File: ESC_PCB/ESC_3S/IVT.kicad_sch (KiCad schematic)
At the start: 45 parts, among them Q1 CSD18532Q5BT, Q2 CSD18532Q5BT, Q3 CSD18532Q5BT, Q4 CSD18532Q5BT, Q5 CSD18532Q5BT, Q6 CSD18532Q5BT, U4 FD6288Q

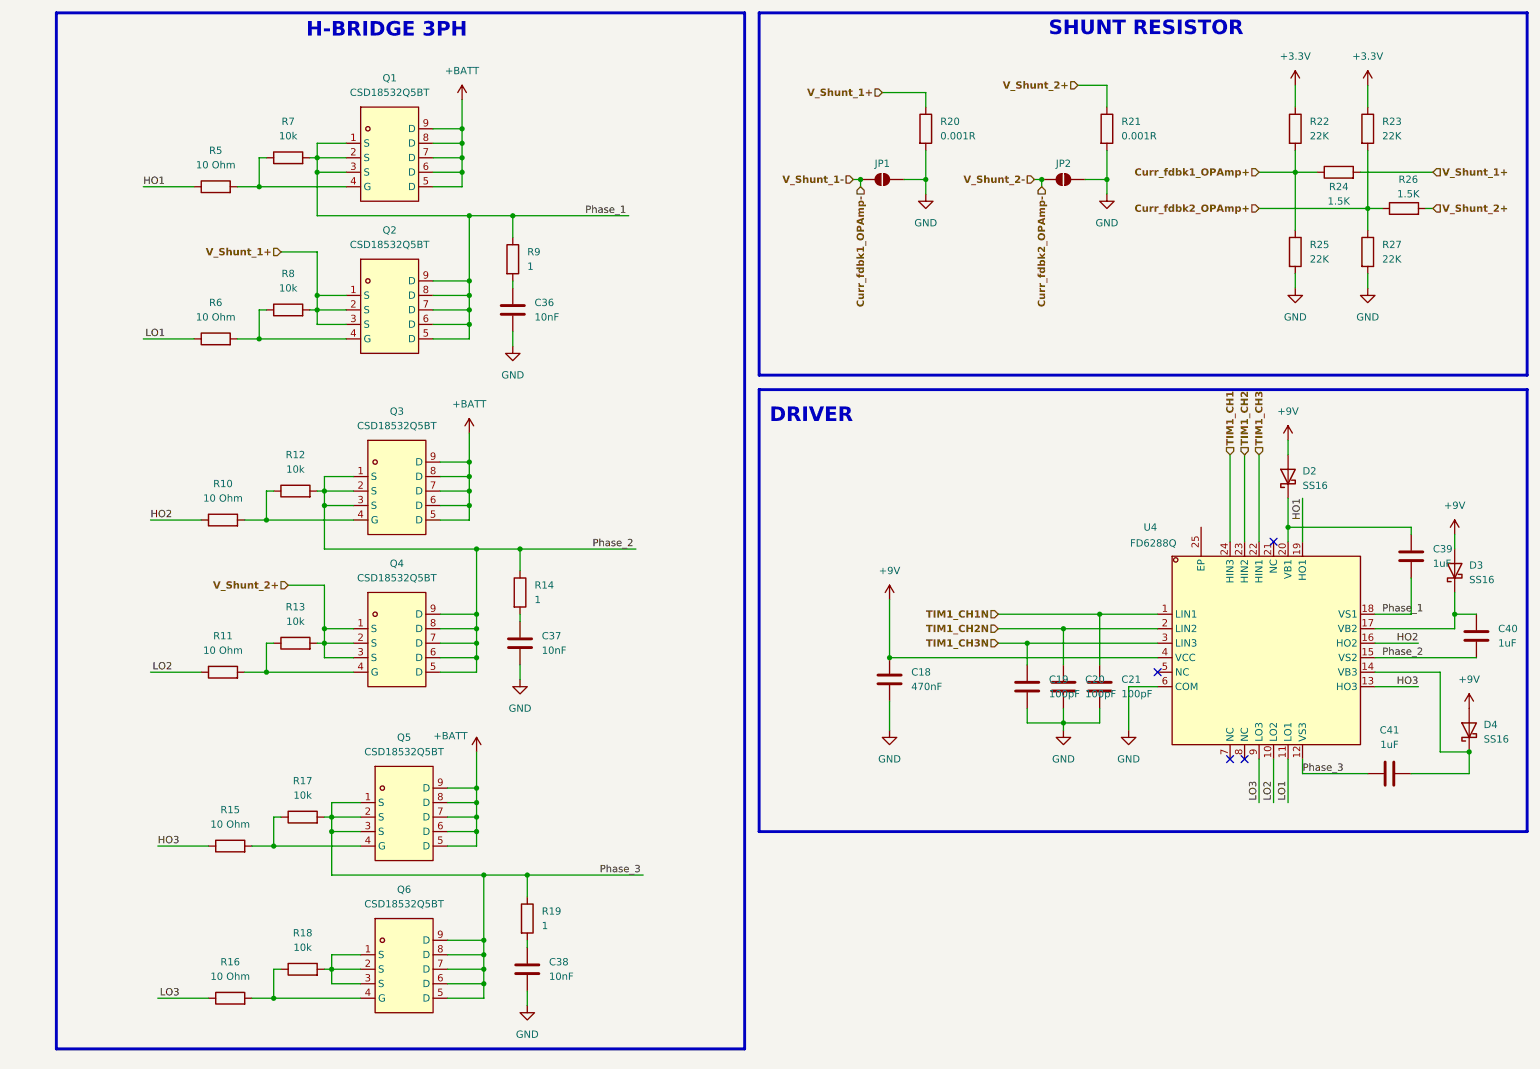
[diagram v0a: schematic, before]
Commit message: add .ioc and temperature done sch
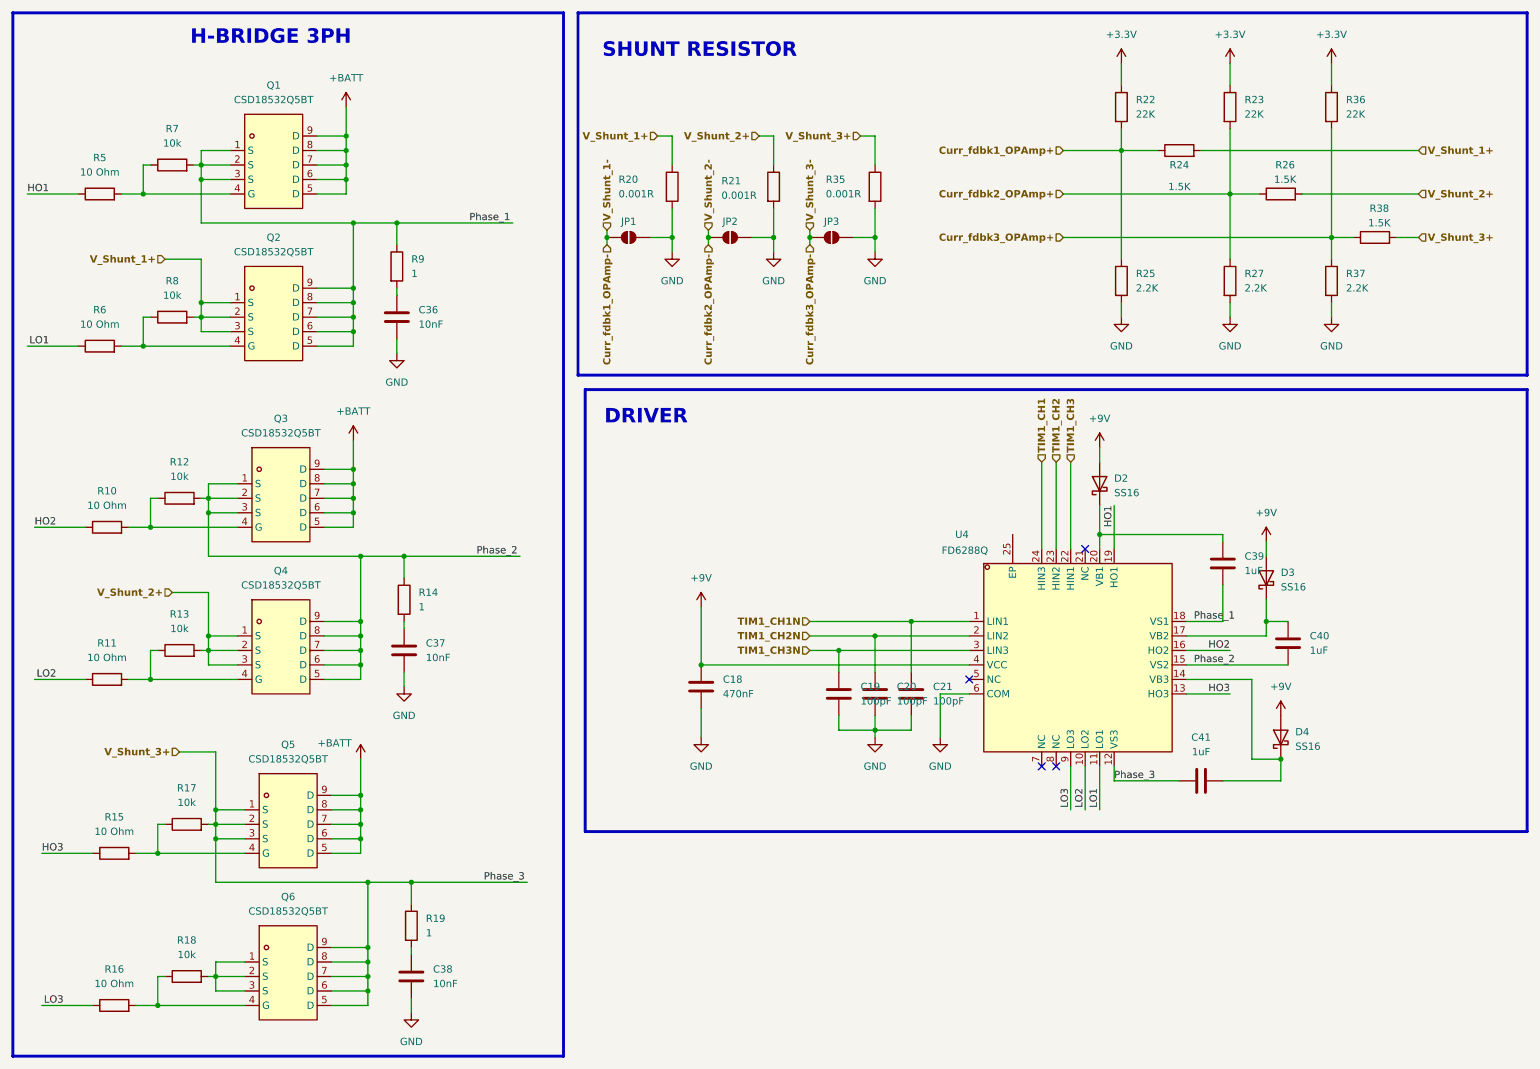
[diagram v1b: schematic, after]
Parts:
- added JP3: SolderJumper_2_Open, Jumper:SolderJumper-2_P1.3mm_Open_TrianglePad1.0x1.5mm, symbol Jumper:SolderJumper_2_Open
- added R35: 0.001R, Resistor_SMD:R_2512_6332Metric_Pad1.40x3.35mm_HandSolder, symbol Device:R
- added R36: 22K, Resistor_SMD:R_0603_1608Metric_Pad0.98x0.95mm_HandSolder, symbol Device:R
- added R37: 2.2K, Resistor_SMD:R_0603_1608Metric_Pad0.98x0.95mm_HandSolder, symbol Device:R
- added R38: 1.5K, Resistor_SMD:R_0603_1608Metric_Pad0.98x0.95mm_HandSolder, symbol Device:R
- R25, R27: value 22K -> 2.2K
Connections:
- net +3.3V: now also R36.1
- net GND: now also JP3.2 (B), R35.2, R37.2
- net Phase_3 renamed V_Shunt_3+
- net V_Shunt_3+: now also R35.1, R38.2
- new net Curr_fdbk3_OPAmp+: R36.2, R37.1, R38.1
- new net Curr_fdbk3_OPAmp-: JP3.1 (A)
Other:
- moved on the sheet: C18, C19, C20, C21, C36, C37, C38, C39, C40, C41, D2, D3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
